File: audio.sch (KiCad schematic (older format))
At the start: 14 parts, among them J12 Audio-Jack-3, U6 PCM5141

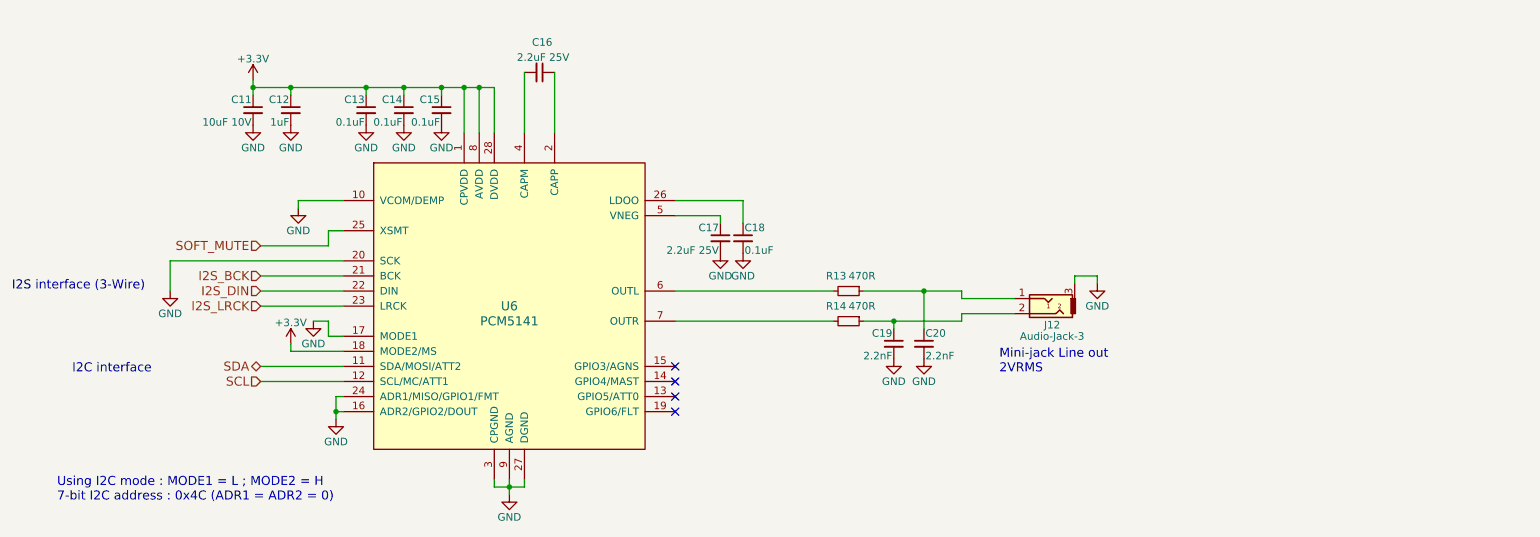
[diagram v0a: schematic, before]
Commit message: Almost all components placed... Saving before mirroring everything
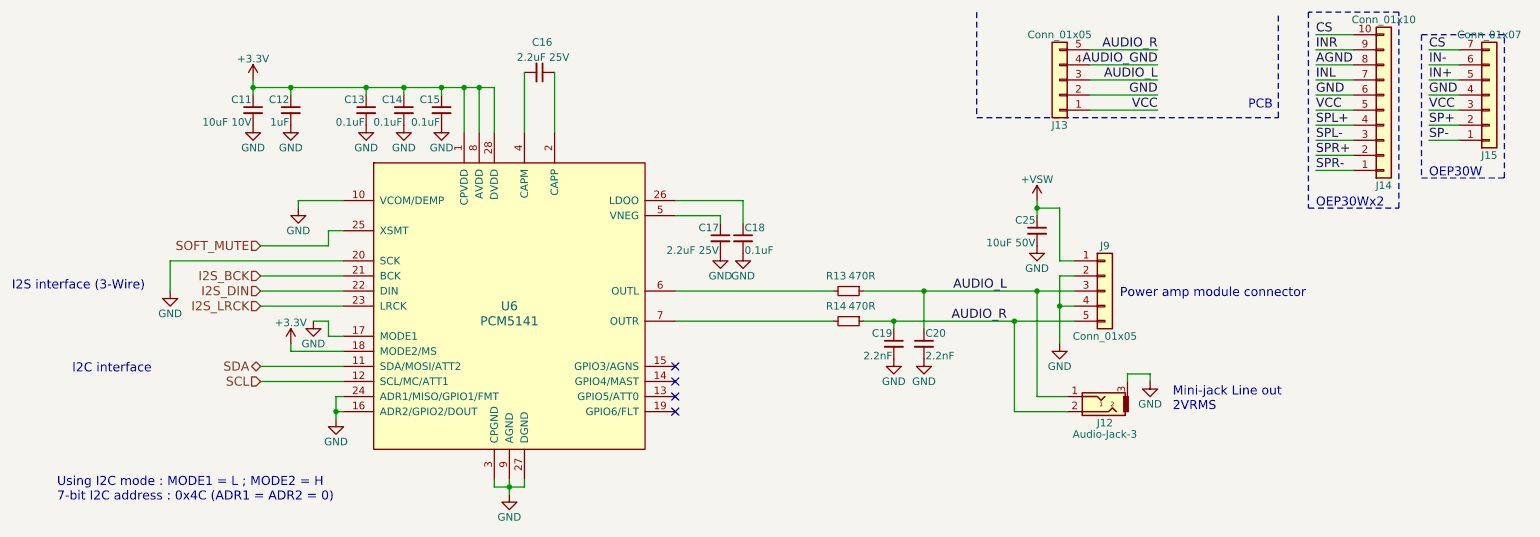
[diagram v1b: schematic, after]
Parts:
- added C25: 10uF 50V, Capacitors_SMD:C_1206, symbol C_Small
- added J13: Conn_01x05, symbol Conn_01x05
- added J14: Conn_01x10, symbol Conn_01x10
- added J15: Conn_01x07, symbol Conn_01x07
- added J9: Conn_01x05, Socket_Strips:Socket_Strip_Straight_1x05_Pitch2.54mm, symbol Conn_01x05
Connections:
- net GND: now also C25.2, J13.2 (Pin_2), J14.6 (Pin_6), J15.4 (Pin_4), J9.2 (Pin_2), J9.4 (Pin_4)
- net AUDIO_L: now reaches C20.1, J12.1, R13.1
- net AUDIO_L: now also J13.3 (Pin_3), J9.3 (Pin_3)
- net AUDIO_R: now reaches C19.1, J12.2, R14.1
- net AUDIO_R: now also J13.5 (Pin_5), J9.5 (Pin_5)
- new net +VSW: C25.1, J9.1 (Pin_1)
- new net AGND: J14.8 (Pin_8)
- new net AUDIO_GND: J13.4 (Pin_4)
- new net CS: J14.10 (Pin_10), J15.7 (Pin_7)
- new net IN+: J15.5 (Pin_5)
- new net IN-: J15.6 (Pin_6)
- new net INL: J14.7 (Pin_7)
- new net INR: J14.9 (Pin_9)
- new net SP+: J15.2 (Pin_2)
- new net SP-: J15.1 (Pin_1)
- new net SPL+: J14.4 (Pin_4)
- new net SPL-: J14.3 (Pin_3)
- new net SPR+: J14.2 (Pin_2)
- new net SPR-: J14.1 (Pin_1)
- new net VCC: J13.1 (Pin_1), J14.5 (Pin_5), J15.3 (Pin_3)
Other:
- note added: "OEP30W"
- note added: "OEP30Wx2"
- note added: "PCB"
- note added: "Power amp module connector"
- moved on the sheet: J12
